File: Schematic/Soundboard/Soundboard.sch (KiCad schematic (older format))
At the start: 0 parts

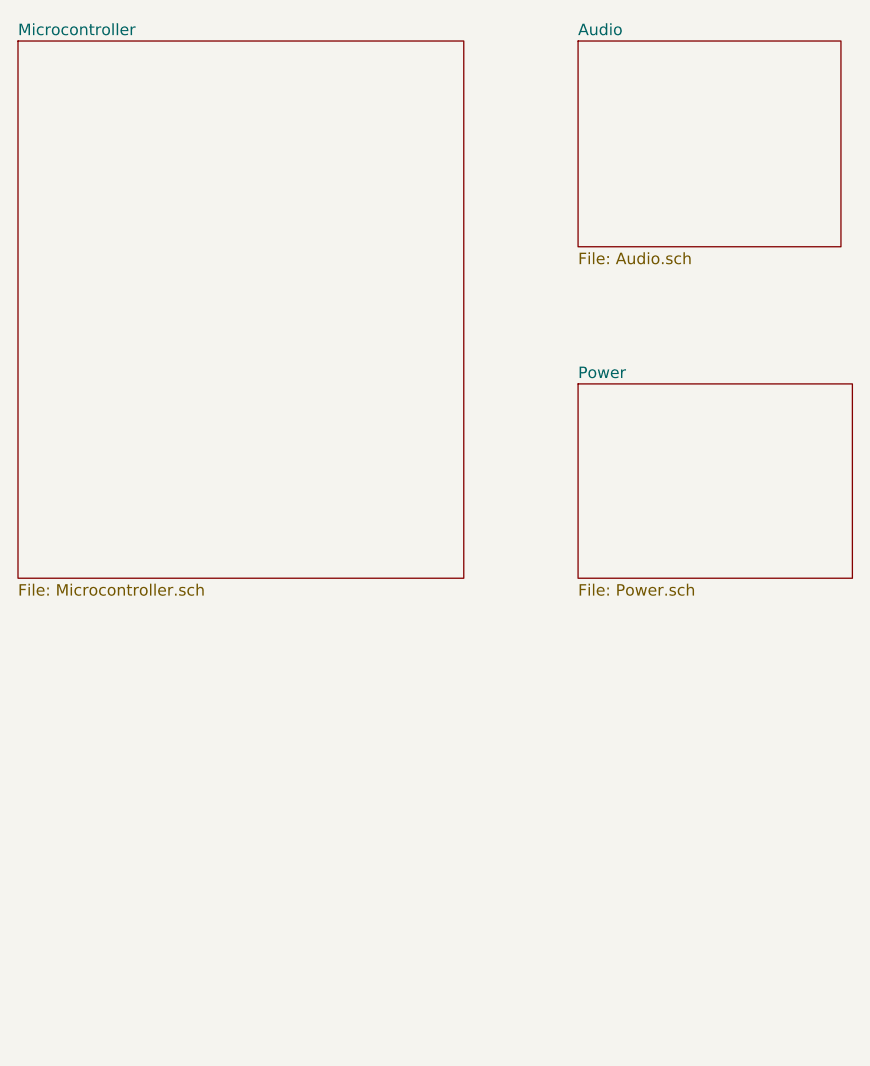
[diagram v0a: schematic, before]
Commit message: Begin rev 2 part selection and schematic
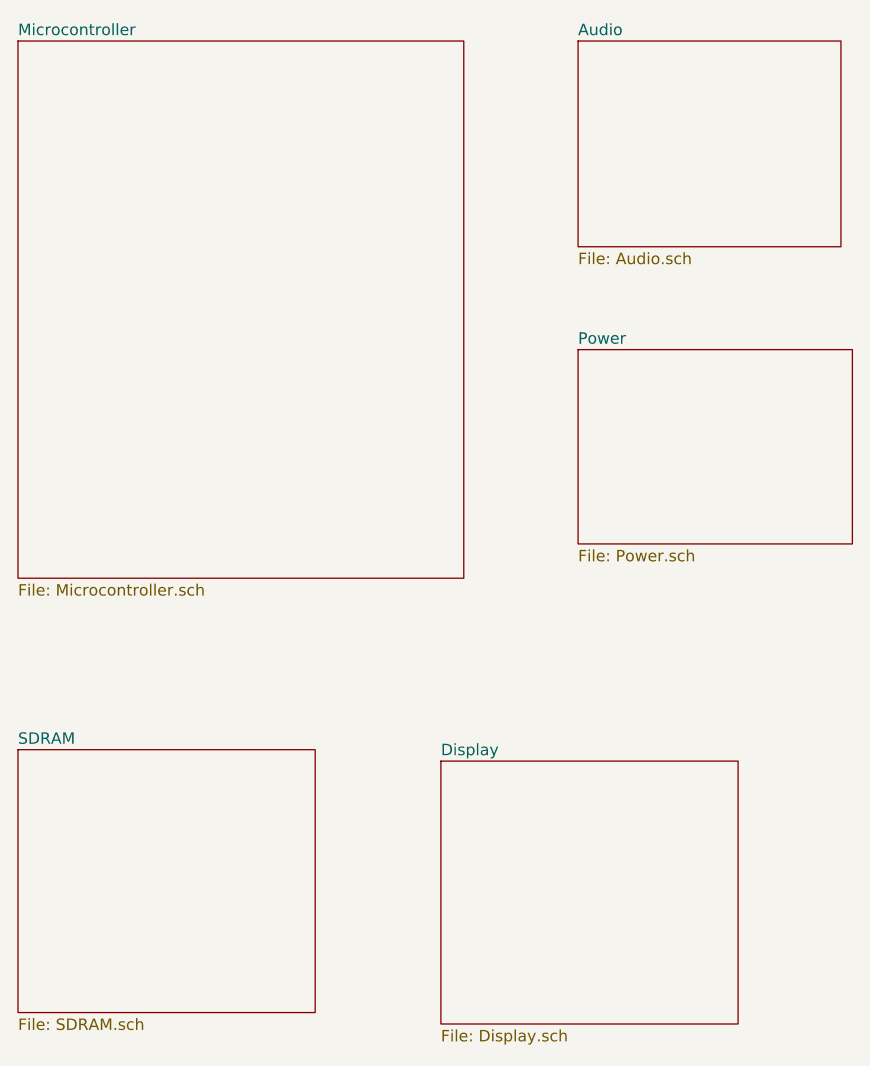
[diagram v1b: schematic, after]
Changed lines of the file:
@@
 $Descr A4 11693 8268
 encoding utf-8
-Sheet 1 4
+Sheet 1 6
 Title ""
 Date ""
@@
 $EndSheet
 $Sheet
-S 4000 3200 1200 850
+S 4000 3050 1200 850
 U 5F0E4BAF
 F0 "Power" 50
 F1 "Power.sch" 50
 $EndSheet
+$Sheet
+S 1550 4800 1300 1150
+U 5F230DA4
+F0 "SDRAM" 50
+F1 "SDRAM.sch" 50
+$EndSheet
+$Sheet
+S 3400 4850 1300 1150
+U 5F230EC3
+F0 "Display" 50
+F1 "Display.sch" 50
+$EndSheet
 $EndSCHEMATC
